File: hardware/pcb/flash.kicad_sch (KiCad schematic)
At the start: 4 parts, among them U7 IS25WP256D-JLLE

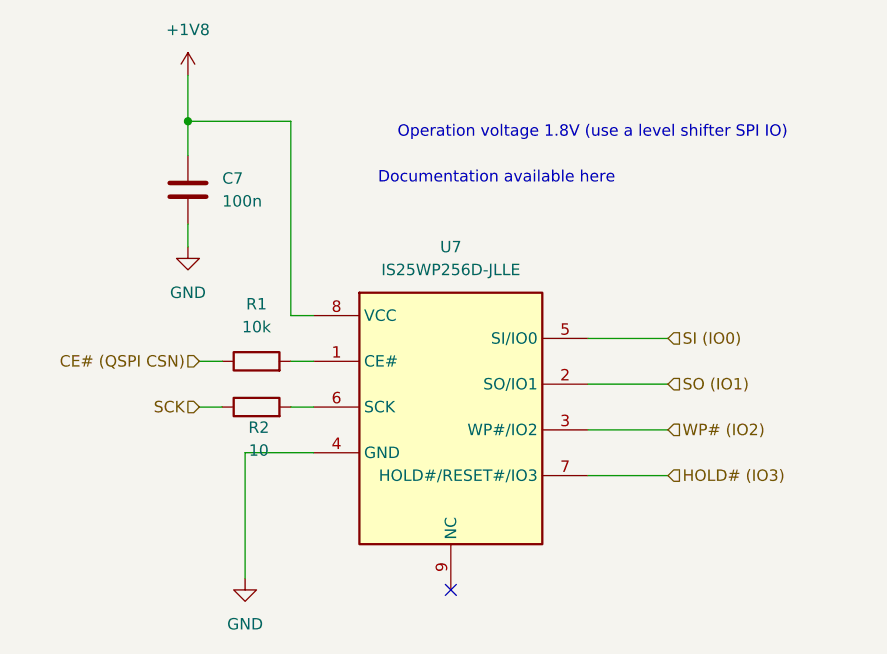
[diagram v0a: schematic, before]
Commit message: Update(hardware): Added new flash symbol
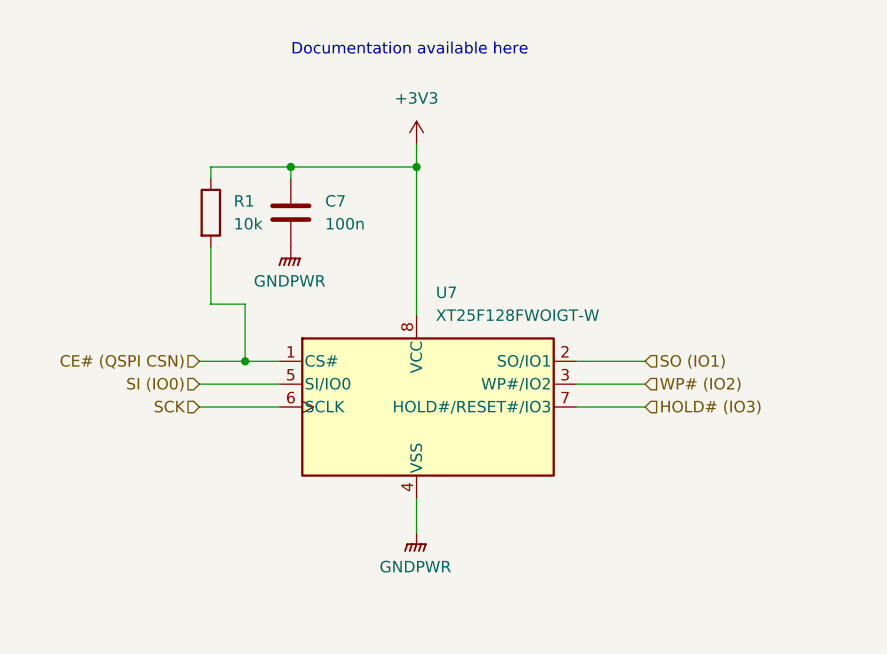
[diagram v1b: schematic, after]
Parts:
- removed R2: 10, symbol Device:R
- removed U7: IS25WP256D-JLLE, Package_SON:WSON-8-1EP_6x5mm_P1.27mm_EP3.4x4.3mm, symbol IS25WP256D-JLLE:IS25WP256D-JLLE
- added U7: XT25F128FWOIGT-W, Package_SON:WSON-8-1EP_6x5mm_P1.27mm_EP3.4x4mm, symbol XT25F128F:XT25F128FWOIGT-W
- C7: footprint Package_SON:WSON-8-1EP_6x5mm_P1.27mm_EP3.4x4.3mm -> Package_SO:SOIC-8_3.9x4.9mm_P1.27mm
- R1: footprint Package_SON:WSON-8-1EP_6x5mm_P1.27mm_EP3.4x4.3mm -> (none)
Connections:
- net CE# (QSPI CSN): now also R1.2, U7.1 (CS#); no longer R1.1
- net HOLD# (IO3): now also U7.7 (HOLD#/RESET#/IO3)
- net SCK: now also U7.6 (SCLK)
- net SI (IO0): now also U7.5 (SI/IO0)
- net SO (IO1): now also U7.2 (SO/IO1)
- net WP# (IO2): now also U7.3 (WP#/IO2)
- net +1V8 renamed +3V3
- net +3V3: now also R1.1, U7.8 (VCC)
- net GND renamed GNDPWR
- net GNDPWR: now also U7.4 (VSS)
- no-connect marks 1 -> 0
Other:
- note removed: "Operation voltage 1.8V (use a level shifter SPI IO)"
